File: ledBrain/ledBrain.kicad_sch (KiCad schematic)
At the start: 44 parts, among them CN1 XT30PW-M, SW1 EC11E09244BS, SW2 K2-1112SW-A4SW-04, U1 QuinLED-ESP32, U10 HS96L03W2C03, U2 MSM261DGT003, U3 CH224A, U4 ME3116, U5 SN74AHCT32QPWRQ1, U7 T34069, U8 T34069, U9 T34069

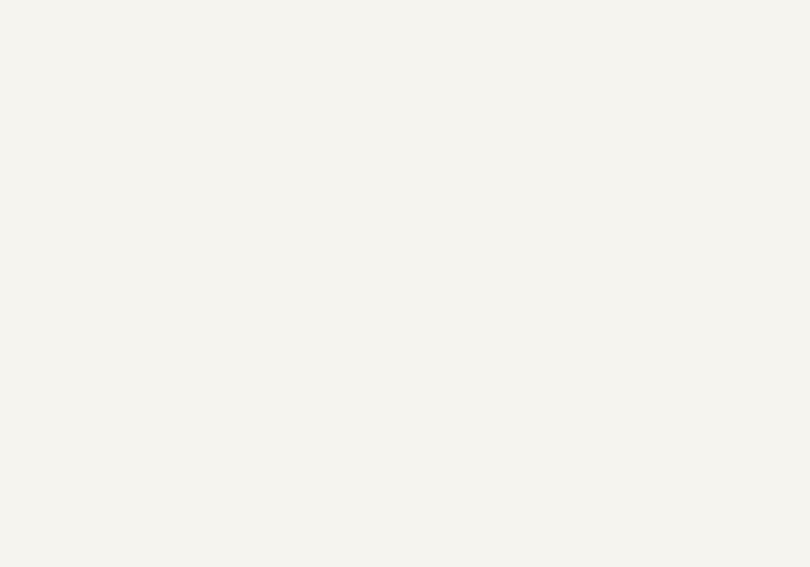
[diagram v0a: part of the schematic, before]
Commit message: update stuff a little bit
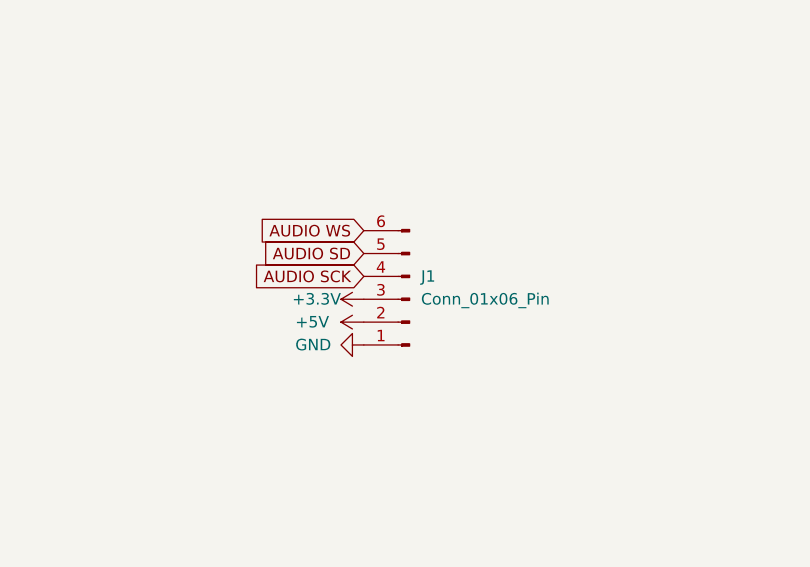
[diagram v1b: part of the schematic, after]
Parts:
- added J1: Conn_01x06_Pin, Connector_PinHeader_2.54mm:PinHeader_1x06_P2.54mm_Vertical, symbol Connector:Conn_01x06_Pin
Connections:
- net +3.3V: now also J1.3 (Pin_3)
- net +5V: now also J1.2 (Pin_2)
- net AUDIO SCK: now also J1.4 (Pin_4)
- net AUDIO SD: now also J1.5 (Pin_5)
- net AUDIO WS: now also J1.6 (Pin_6)
- net GND: now also J1.1 (Pin_1)
